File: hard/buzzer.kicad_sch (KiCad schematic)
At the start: 3 parts, among them Q1 DTD123Y

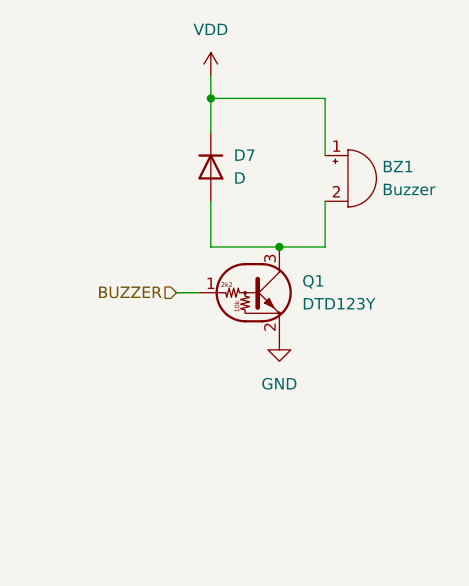
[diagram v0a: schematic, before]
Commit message: update
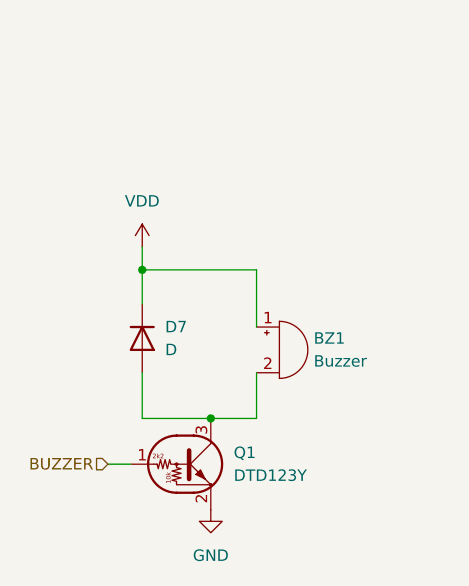
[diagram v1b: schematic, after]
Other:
- moved on the sheet: BZ1, D7, Q1
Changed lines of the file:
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@@
 	(paper "A4")
 	(junction
-		(at 149.86 63.5)
+		(at 142.24 82.55)
 		(diameter 0)
 		(color 0 0 0 0)
 	)
 	(junction
-		(at 157.48 80.01)
+		(at 149.86 99.06)
 		(diameter 0)
 		(color 0 0 0 0)
@@
 	(wire
 		(pts
-			(xy 149.86 80.01) (xy 149.86 74.93)
-		)
-		(stroke
-			(width 0)
-			(type default)
-		)
-	)
-	(wire
-		(pts
-			(xy 149.86 63.5) (xy 149.86 67.31)
-		)
-		(stroke
-			(width 0)
-			(type default)
-		)
-	)
-	(wire
-		(pts
-			(xy 162.56 74.93) (xy 162.56 80.01)
-		)
-		(stroke
-			(width 0)
-			(type default)
-		)
-	)
-	(wire
-		(pts
-			(xy 162.56 63.5) (xy 149.86 63.5)
-		)
-		(stroke
-			(width 0)
-			(type default)
-		)
-	)
-	(wire
-		(pts
-			(xy 149.86 60.96) (xy 149.86 63.5)
-		)
-		(stroke
-			(width 0)
-			(type default)
-		)
-	)
-	(wire
-		(pts
-			(xy 157.48 80.01) (xy 149.86 80.01)
-		)
-		(stroke
-			(width 0)
-			(type default)
-		)
-	)
-	(wire
-		(pts
-			(xy 162.56 69.85) (xy 162.56 63.5)
-		)
-		(stroke
-			(width 0)
-			(type default)
-		)
-	)
-	(wire
-		(pts
-			(xy 162.56 80.01) (xy 157.48 80.01)
-		)
-		(stroke
-			(width 0)
-			(type default)
-		)
-	)
-	(wire
-		(pts
-			(xy 146.05 85.09) (xy 148.59 85.09)
+			(xy 142.24 99.06) (xy 142.24 93.98)
+		)
+		(stroke
+			(width 0)
+			(type default)
+		)
+	)
+	(wire
+		(pts
+			(xy 142.24 82.55) (xy 142.24 86.36)
+		)
+		(stroke
+			(width 0)
+			(type default)
+		)
+	)
+	(wire
+		(pts
+			(xy 154.94 93.98) (xy 154.94 99.06)
+		)
+		(stroke
+			(width 0)
+			(type default)
+		)
+	)
+	(wire
+		(pts
+			(xy 154.94 82.55) (xy 142.24 82.55)
+		)
+		(stroke
+			(width 0)
+			(type default)
+		)
+	)
+	(wire
+		(pts
+			(xy 142.24 80.01) (xy 142.24 82.55)
+		)
+		(stroke
+			(width 0)
+			(type default)
+		)
+	)
+	(wire
+		(pts
+			(xy 149.86 99.06) (xy 142.24 99.06)
+		)
+		(stroke
+			(width 0)
+			(type default)
+		)
+	)
+	(wire
+		(pts
+			(xy 154.94 88.9) (xy 154.94 82.55)
+		)
+		(stroke
+			(width 0)
+			(type default)
+		)
+	)
+	(wire
+		(pts
+			(xy 154.94 99.06) (xy 149.86 99.06)
+		)
+		(stroke
+			(width 0)
+			(type default)
+		)
+	)
+	(wire
+		(pts
+			(xy 138.43 104.14) (xy 140.97 104.14)
 		)
 		(stroke
@@
 	(hierarchical_label "BUZZER"
 		(shape input)
-		(at 146.05 85.09 180)
+		(at 138.43 104.14 180)
 		(effects
 			(font
@@
 	(symbol
 		(lib_id "Device:D")
-		(at 149.86 71.12 270)
+		(at 142.24 90.17 270)
 		(unit 1)
 		(exclude_from_sim no)
@@
 		(fields_autoplaced yes)
 		(property "Reference" "D7"
-			(at 152.4 69.8499 90)
+			(at 144.78 88.8999 90)
 			(effects
 				(font
@@
 		)
 		(property "Value" "D"
-			(at 152.4 72.3899 90)
+			(at 144.78 91.4399 90)
 			(effects
 				(font
@@
 		)
 		(property "Footprint" ""
-			(at 149.86 71.12 0)
+			(at 142.24 90.17 0)
 			(effects
 				(font
@@
 		)
 		(property "Datasheet" "~"
-			(at 149.86 71.12 0)
+			(at 142.24 90.17 0)
 			(effects
 				(font
@@
 		)
 		(property "Description" "Diode"
-			(at 149.86 71.12 0)
+			(at 142.24 90.17 0)
 			(effects
 				(font
@@
 		)
 		(property "Sim.Device" "D"
-			(at 149.86 71.12 0)
+			(at 142.24 90.17 0)
 			(effects
 				(font
@@
 		)
 		(property "Sim.Pins" "1=K 2=A"
-			(at 149.86 71.12 0)
+			(at 142.24 90.17 0)
 			(effects
 				(font
@@
 	(symbol
 		(lib_id "Device:Buzzer")
-		(at 165.1 72.39 0)
+		(at 157.48 91.44 0)
 		(unit 1)
 		(exclude_from_sim no)
@@
 		(on_board yes)
 		(dnp no)
-		(fields_autoplaced yes)
 		(property "Reference" "BZ1"
-			(at 168.91 71.1199 0)
+			(at 161.29 90.1699 0)
 			(effects
 				(font
@@
 		)
 		(property "Value" "Buzzer"
-			(at 168.91 73.6599 0)
+			(at 161.29 92.7099 0)
 			(effects
 				(font
@@
 		)
 		(property "Footprint" ""
-			(at 164.465 69.85 90)
+			(at 156.845 88.9 90)
 			(effects
 				(font
@@
 		)
 		(property "Datasheet" "~"
-			(at 164.465 69.85 90)
+			(at 156.845 88.9 90)
 			(effects
 				(font
@@
 		)
 		(property "Description" "Buzzer, polarized"
-			(at 165.1 72.39 0)
+			(at 157.48 91.44 0)
 			(effects
 				(font
@@
 	(symbol
 		(lib_id "Transistor_BJT:DTD123Y")
-		(at 154.94 85.09 0)
+		(at 147.32 104.14 0)
 		(unit 1)
 		(exclude_from_sim no)
@@
 		(fields_autoplaced yes)
 		(property "Reference" "Q1"
-			(at 160.02 83.8199 0)
+			(at 152.4 102.8699 0)
 			(effects
 				(font
@@
 		)
 		(property "Value" "DTD123Y"
-			(at 160.02 86.3599 0)
+			(at 152.4 105.4099 0)
 			(effects
 				(font
@@
 		)
 		(property "Footprint" ""
-			(at 154.94 85.09 0)
+			(at 147.32 104.14 0)
 			(effects
 				(font
@@
 		)
 		(property "Datasheet" ""
-			(at 154.94 85.09 0)
+			(at 147.32 104.14 0)
 			(effects
 				(font
@@
 		)
 		(property "Description" "Digital NPN Transistor, 2k2/10k, SOT-23"
-			(at 154.94 85.09 0)
+			(at 147.32 104.14 0)
 			(effects
 				(font
@@
 	(symbol
 		(lib_id "power:VDD")
-		(at 149.86 60.96 0)
+		(at 142.24 80.01 0)
 		(unit 1)
 		(exclude_from_sim no)
@@
 		(dnp no)
 		(property "Reference" "#PWR048"
-			(at 149.86 64.77 0)
+			(at 142.24 83.82 0)
 			(effects
 				(font
@@
 		)
 		(property "Value" "VDD"
-			(at 149.86 55.88 0)
+			(at 142.24 74.93 0)
 			(effects
 				(font
@@
 		)
 		(property "Footprint" ""
-			(at 149.86 60.96 0)
+			(at 142.24 80.01 0)
 			(effects
 				(font
@@
 		)
 		(property "Datasheet" ""
-			(at 149.86 60.96 0)
+			(at 142.24 80.01 0)
 			(effects
 				(font
@@
 		)
 		(property "Description" "Power symbol creates a global label with name \"VDD\""
-			(at 149.86 60.96 0)
+			(at 142.24 80.01 0)
 			(effects
 				(font
@@
 	(symbol
 		(lib_id "power:GND")
-		(at 157.48 90.17 0)
+		(at 149.86 109.22 0)
 		(unit 1)
 		(exclude_from_sim no)
@@
 		(fields_autoplaced yes)
 		(property "Reference" "#PWR049"
-			(at 157.48 96.52 0)
+			(at 149.86 115.57 0)
 			(effects
 				(font
@@
 		)
 		(property "Value" "GND"
-			(at 157.48 95.25 0)
+			(at 149.86 114.3 0)
 			(effects
 				(font
@@
 		)
 		(property "Footprint" ""
-			(at 157.48 90.17 0)
+			(at 149.86 109.22 0)
 			(effects
 				(font
@@
 		)
 		(property "Datasheet" ""
-			(at 157.48 90.17 0)
+			(at 149.86 109.22 0)
 			(effects
 				(font
@@
 		)
 		(property "Description" "Power symbol creates a global label with name \"GND\" , ground"
-			(at 157.48 90.17 0)
-			(effects
-				(font
+			(at 149.86 109.22 0)
+			(effects
+				(font
